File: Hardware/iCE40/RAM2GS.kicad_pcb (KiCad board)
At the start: 4 copper layers, 67.3 x 48.5 mm, 69 parts, among them J1 Memory Expansion, J2 JTAG, U1 iCE40HX1K-VQ100, U10 74LVC1G04GW, U11 AP2127K-1.2TRG1, U12 25F010, U13 AP2127K-2.5TRG1, U2 W9812G6KH-6, U3 60M, U4 74AHCT245PW, U5 74LVC245APW, U6 74LVC245APW, U7 74LVC245APW, U8 AZ1117CH-3.3TRG1, U9 74LVC1G04GW

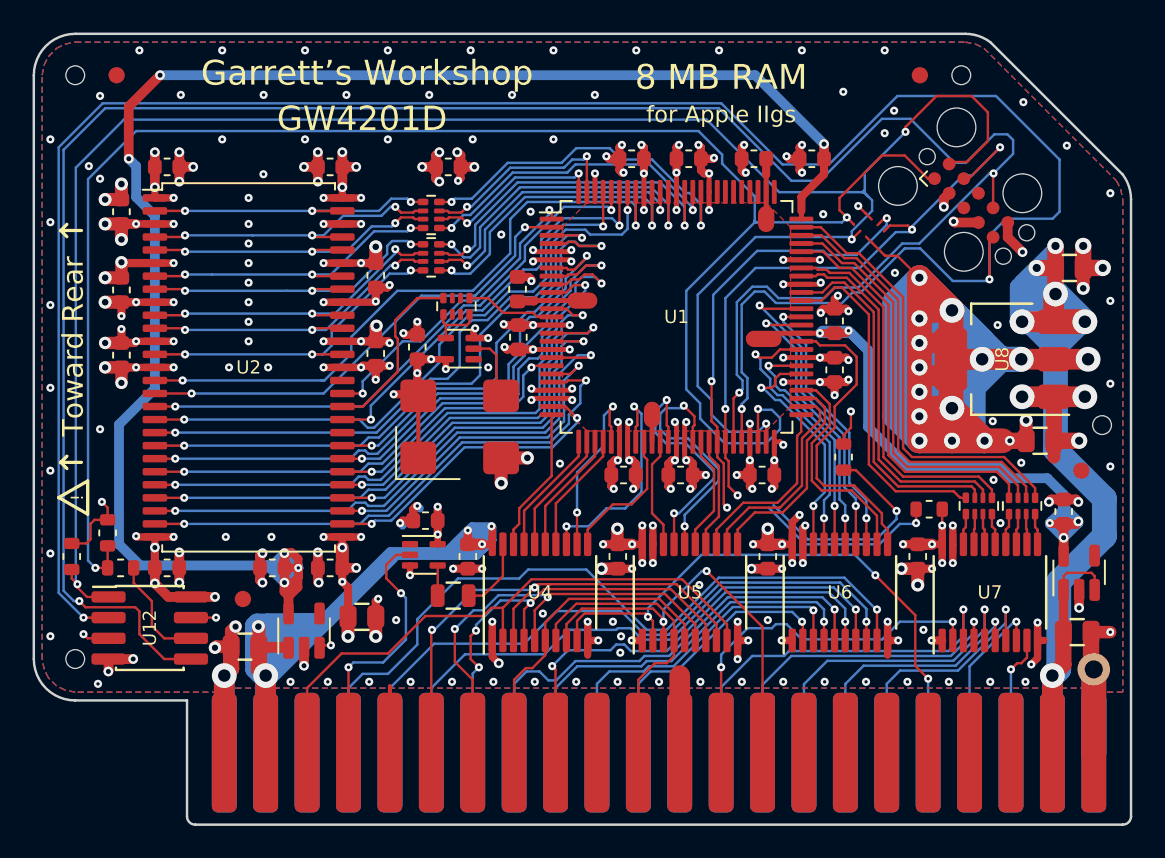
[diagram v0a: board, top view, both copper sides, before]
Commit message: Generated gerbers and documenation PDFs
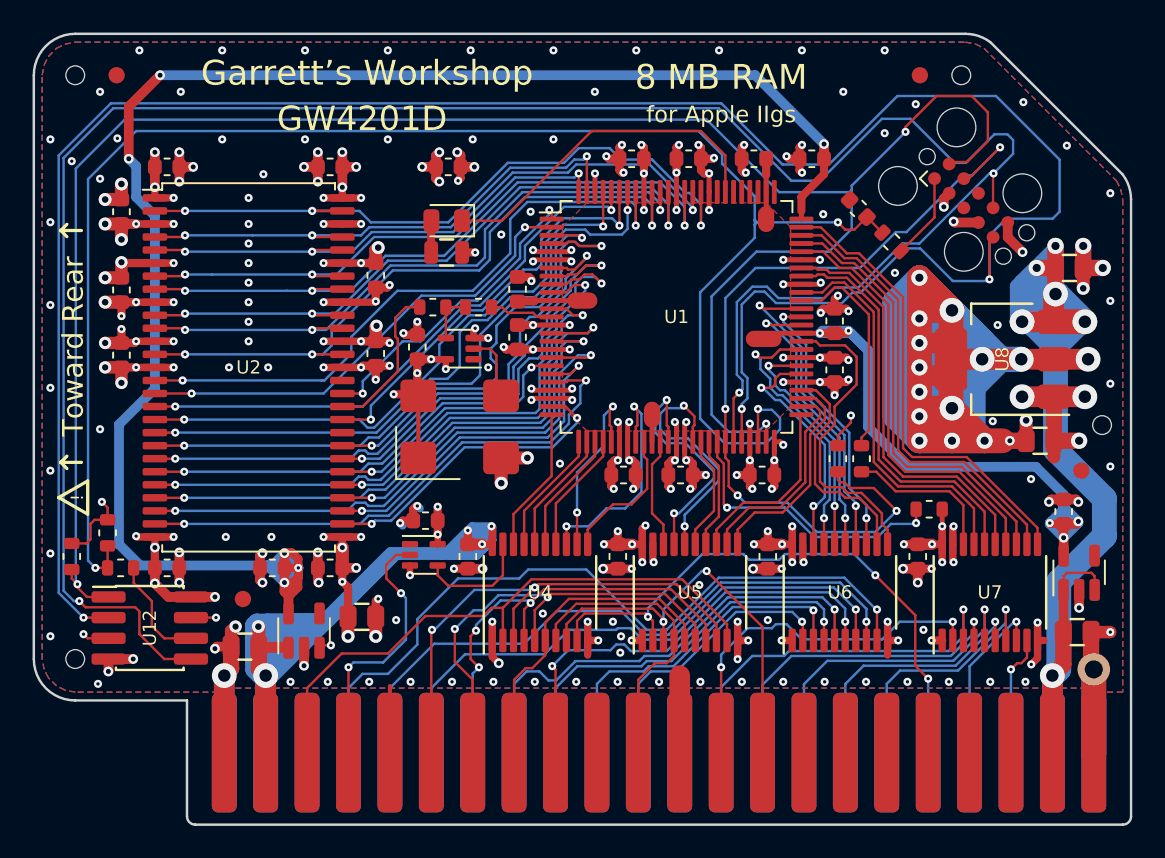
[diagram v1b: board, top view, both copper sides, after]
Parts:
- removed RN1, RN2, RN3, RN4, RN5: 4x33, stdpads:R4_0402
- added C35: 15p, stdpads:C_0603, F.Cu at (96.5, 101.9)
- added D1: White, stdpads:LED_0805, F.Cu at (71.3, 102.7)
- added R10: 47, stdpads:R_0603, F.Cu at (98.6, 104.0)
- added R7: 180, stdpads:R_0805, F.Cu at (71.3, 104.6)
- added R8: 47, stdpads:R_0603, F.Cu at (70.5, 108.0)
- added R9: 47, stdpads:R_0603, F.Cu at (73.2, 108.0)
- J1: value Memory Expansion -> IIgs RAM Exp.
- R1: renamed from R4; value 33 -> 10k
- R2: value 33 -> 47
- R3: value 100 -> 47; footprint stdpads:R_0805 -> stdpads:R_0603
- R4: renamed from R1; value 33 -> 10k
- R5, R6: value 33 -> 10k
- moved R3 26.4 mm to (96.8, 117.2), turned to 270 degrees
- moved R1 0.36 mm to (95.3, 117.2)
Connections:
- J2 pad 1: /CCK -> /CCKr2
- R1 pad 2: /CDONE -> /C~RST~
- R3 pad 1: Net-(R3-Pad1) -> /~CRAS~in
- R4 pad 2: /C~RST~ -> /CDONE
- U1 pad 100: /RD2r -> /RD3
- U1 pad 82: Net-(U1-Pad82) -> /LED
- U1 pad 85: /RD0r -> /RD0
- U1 pad 86: /RD3r -> /RD2
- U1 pad 87: /RD5r -> /RD4
- U1 pad 89: /RD4r -> /RD5
- U1 pad 90: /RD6r -> /RD6
- U1 pad 91: /RD7r -> /RD7
- U1 pad 99: /RD1r -> /RD1
- U4 pad 19: Net-(R3-Pad2) -> Net-(U4-Pad19)
- U7 pad 11: Net-(RN5-Pad4) -> /Ain9
- U7 pad 12: Net-(RN5-Pad3) -> /Ain8
- U7 pad 13: Net-(RN5-Pad2) -> /Ain6
- U7 pad 14: Net-(RN5-Pad1) -> /Ain3
- U7 pad 15: Net-(RN4-Pad4) -> /Ain4
- U7 pad 16: Net-(RN4-Pad3) -> /Ain5
- U7 pad 17: Net-(RN4-Pad2) -> /Ain7
- U7 pad 18: Net-(RN4-Pad1) -> Net-(R3-Pad2)
- U9 pad 4: Net-(R3-Pad1) -> Net-(U4-Pad19)
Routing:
- net /RD0: track 18.6 -> 42.3 mm
- net /CDONE: track 41.0 -> 17.8 mm, vias 4 -> 2
- net /RD0r: track 22.2 -> 0.00 mm, vias 2 -> 0
- net /RD5r: track 21.5 -> 0.00 mm, vias 2 -> 0
- net /LED: track 0.00 -> 21.3 mm
- net /RD4: track 20.0 -> 41.0 mm
- net /RD4r: track 20.7 -> 0.00 mm, vias 2 -> 0
- net /RD7: track 20.8 -> 41.3 mm
- net /RD2: track 19.4 -> 39.6 mm
- net /RD5: track 20.3 -> 40.3 mm
- net /RD3r: track 19.6 -> 0.00 mm, vias 2 -> 0
- net /RD7r: track 19.4 -> 0.00 mm, vias 2 -> 0
- net /RD6: track 20.2 -> 39.2 mm
- net /RD6r: track 18.2 -> 0.00 mm, vias 2 -> 0
- net /RD1: track 19.3 -> 32.6 mm
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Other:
- board text added: "D20D"
